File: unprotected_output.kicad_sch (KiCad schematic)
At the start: 0 parts

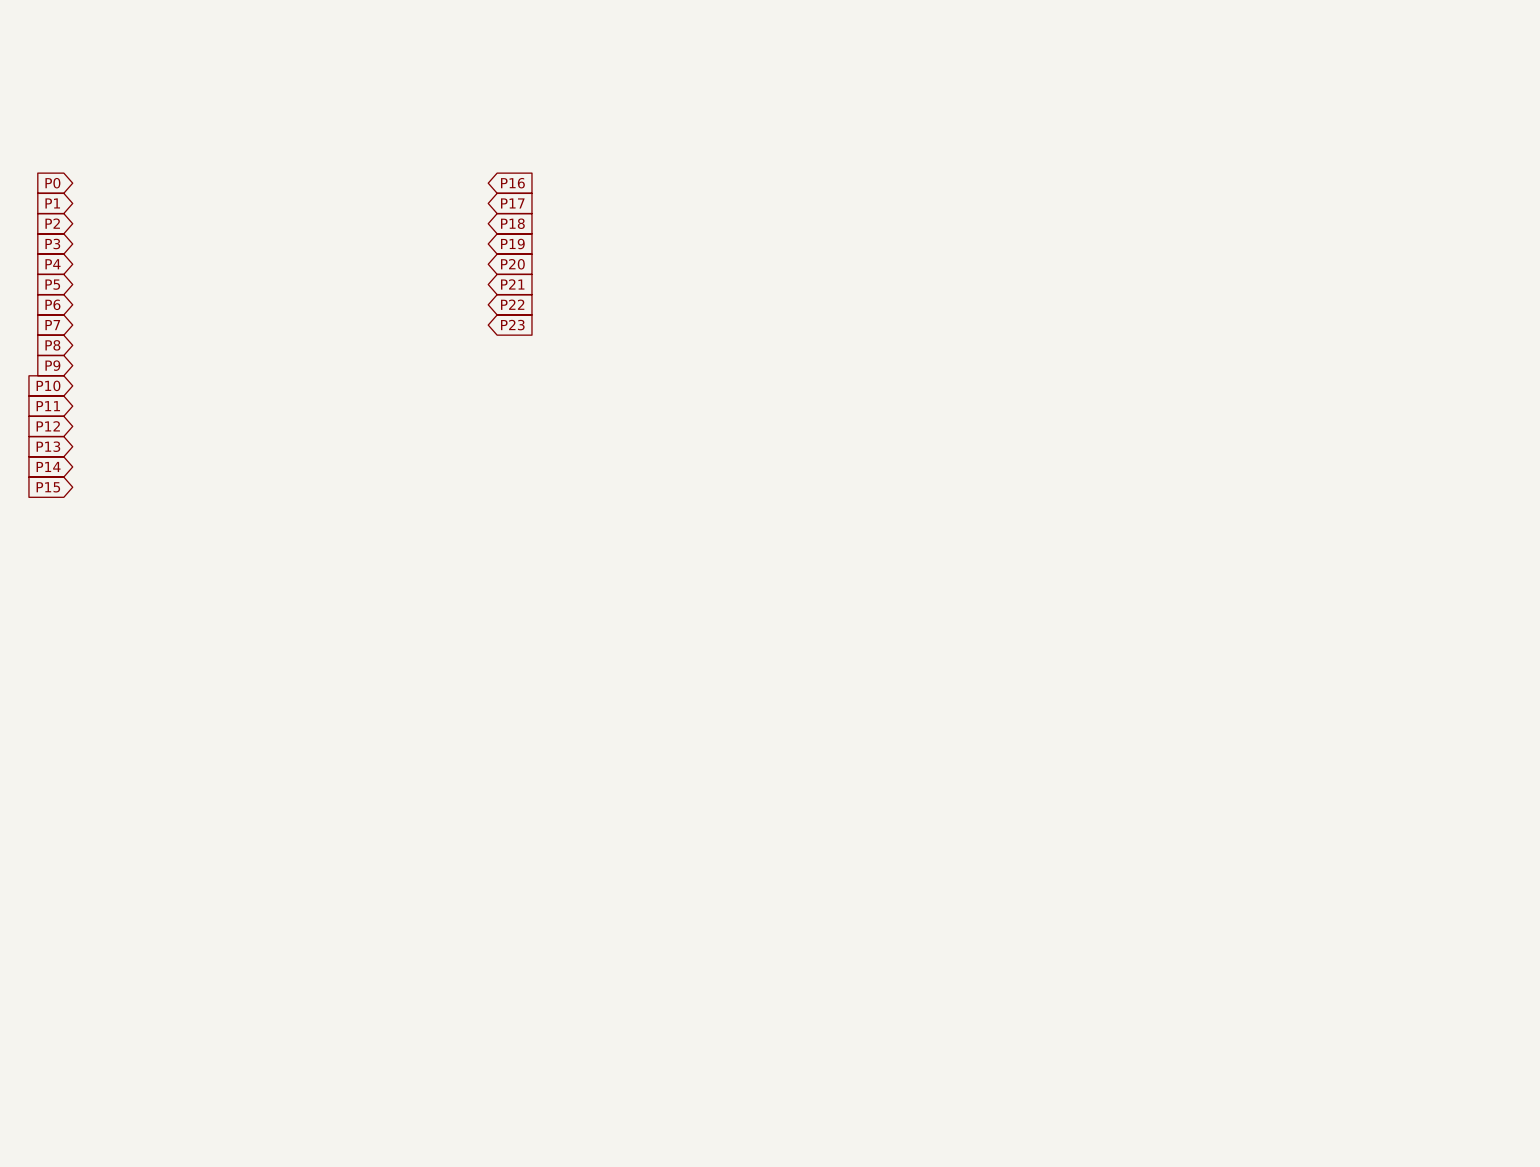
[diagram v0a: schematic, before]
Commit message: [WIP] unprotected front-end sheet with components
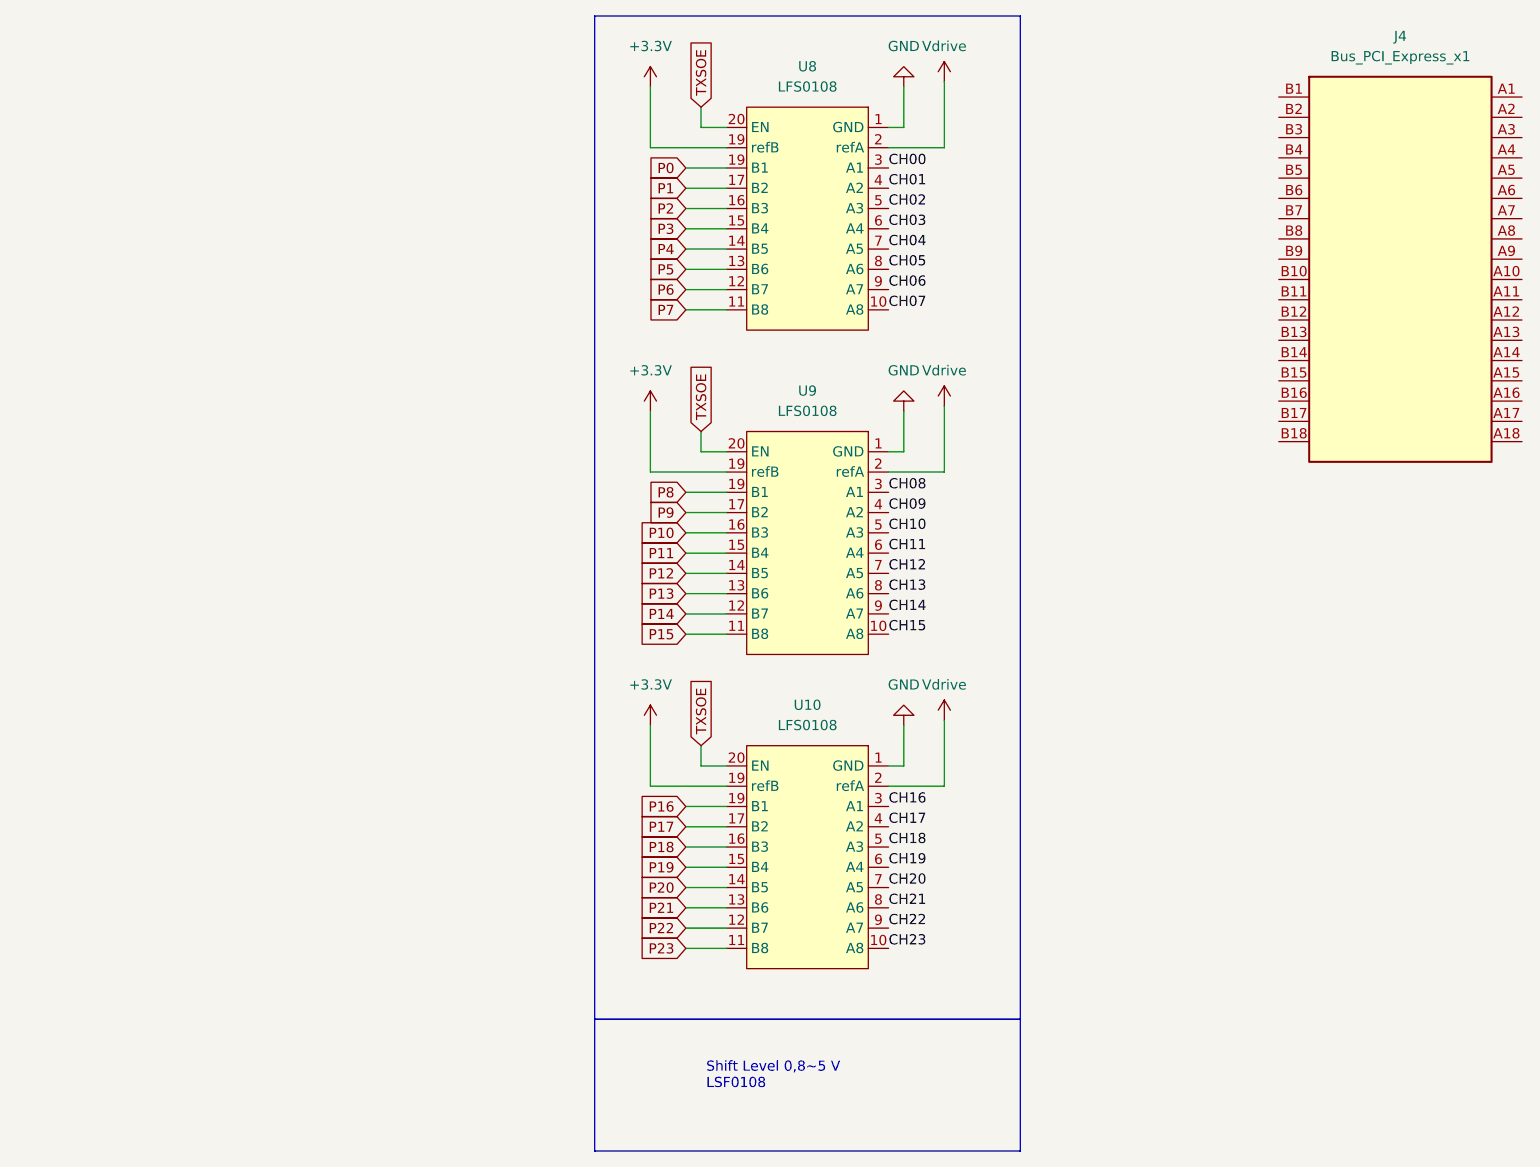
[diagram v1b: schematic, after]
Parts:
- added J4: Bus_PCI_Express_x1, Connector_PCBEdge:BUS_PCIexpress_x1, symbol Connectors:Bus_PCI_Express_x1
- added U10, U8, U9: LFS0108, Package_SO:TSSOP-20_4.4x6.5mm_P0.65mm, symbol Logic_Level_Translator:LSF0108
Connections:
- net P0: now also U8.19 (refB)
- net P1: now also U8.17 (B2)
- net P10: now also U9.16 (B3)
- net P11: now also U9.15 (B4)
- net P12: now also U9.14 (B5)
- net P13: now also U9.13 (B6)
- net P14: now also U9.12 (B7)
- net P15: now also U9.11 (B8)
- net P16: now also U10.19 (refB)
- net P17: now also U10.17 (B2)
- net P18: now also U10.16 (B3)
- net P19: now also U10.15 (B4)
- net P2: now also U8.16 (B3)
- net P20: now also U10.14 (B5)
- net P21: now also U10.13 (B6)
- net P22: now also U10.12 (B7)
- net P23: now also U10.11 (B8)
- net P3: now also U8.15 (B4)
- net P4: now also U8.14 (B5)
- net P5: now also U8.13 (B6)
- net P6: now also U8.12 (B7)
- net P7: now also U8.11 (B8)
- net P8: now also U9.19 (refB)
- net P9: now also U9.17 (B2)
- new net +3.3V: U10.19 (refB), U8.19 (refB), U9.19 (refB)
- new net CH00: U8.3 (A1)
- new net CH01: U8.4 (A2)
- new net CH02: U8.5 (A3)
- new net CH03: U8.6 (A4)
- new net CH04: U8.7 (A5)
- new net CH05: U8.8 (A6)
- new net CH06: U8.9 (A7)
- new net CH07: U8.10 (A8)
- new net CH08: U9.3 (A1)
- new net CH09: U9.4 (A2)
- new net CH10: U9.5 (A3)
- new net CH11: U9.6 (A4)
- new net CH12: U9.7 (A5)
- new net CH13: U9.8 (A6)
- new net CH14: U9.9 (A7)
- new net CH15: U9.10 (A8)
- new net CH16: U10.3 (A1)
- new net CH17: U10.4 (A2)
- new net CH18: U10.5 (A3)
- new net CH19: U10.6 (A4)
- new net CH20: U10.7 (A5)
- new net CH21: U10.8 (A6)
- new net CH22: U10.9 (A7)
- new net CH23: U10.10 (A8)
- new net GND: U10.1 (GND), U8.1 (GND), U9.1 (GND)
- new net TXSOE: U10.20 (EN), U8.20 (EN), U9.20 (EN)
- new net Vdrive: U10.2 (refA), U8.2 (refA), U9.2 (refA)
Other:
- note added: "Shift Level 0,8~5 V LSF0108"
